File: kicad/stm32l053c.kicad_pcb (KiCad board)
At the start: 2 copper layers, 52 x 35 mm, 42 parts, among them P1 SWD, P2 PWR, Q1 BC807, Q2 BC817, SW1 SW_PUSH, SW2 SW_PUSH, SW3 SW_PUSH, U1 STM32L053C8_LQFP48, U2 TLV61225, U3 um66t, Y1 Crystal

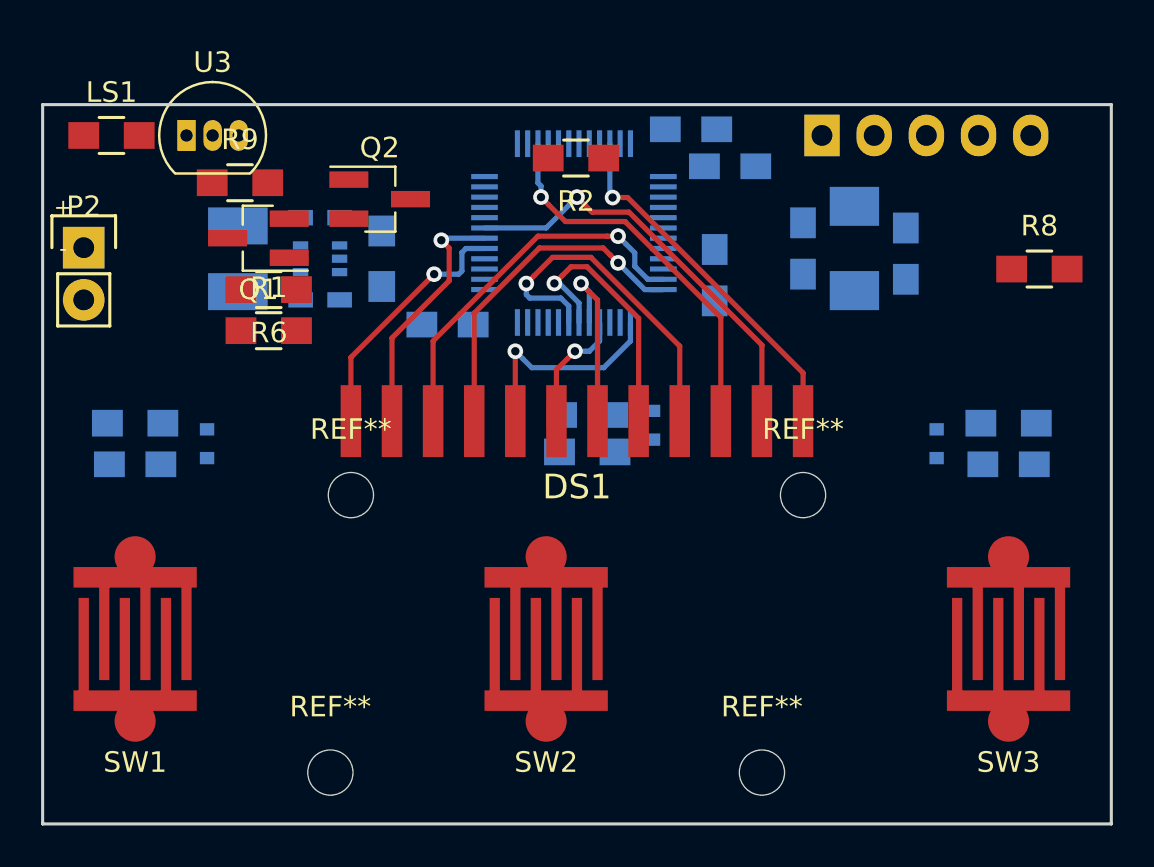
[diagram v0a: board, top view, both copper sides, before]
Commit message: Crystal & melody footprints
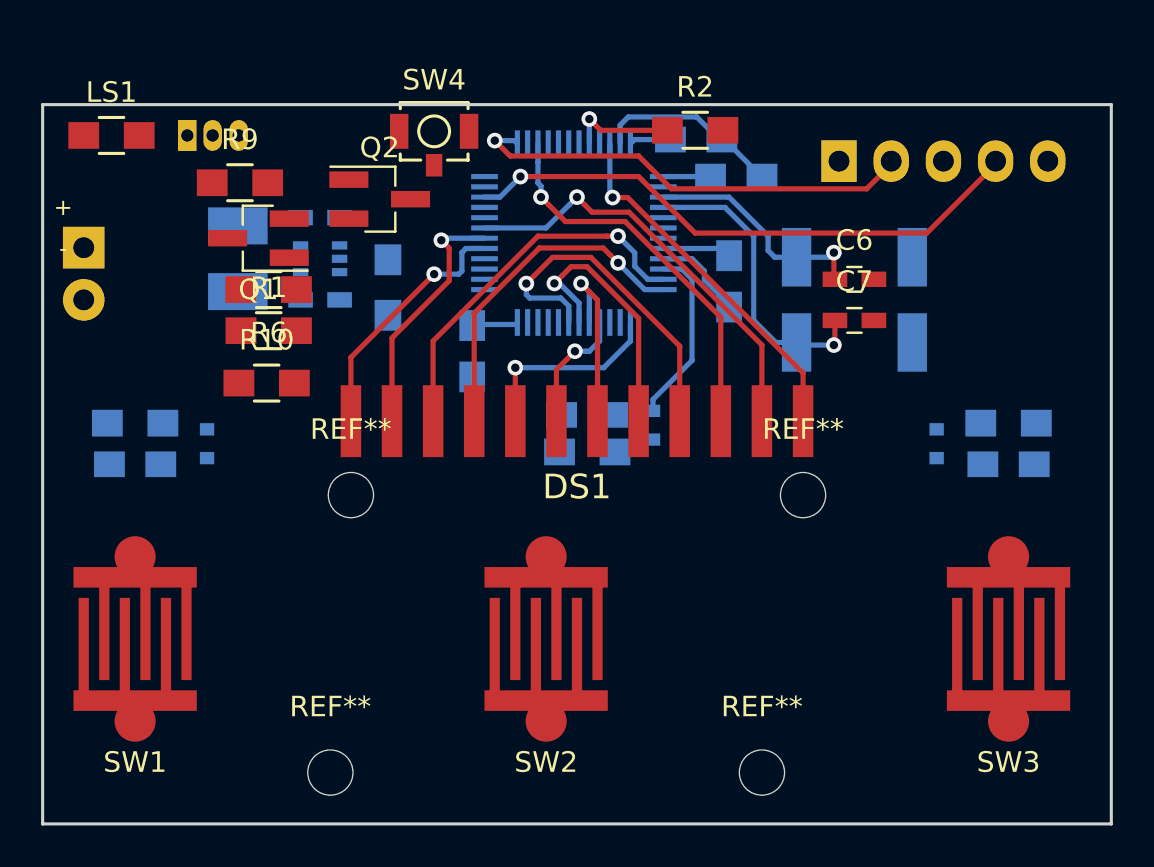
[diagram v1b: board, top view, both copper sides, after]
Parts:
- removed R8: 0, Resistors_SMD:R_0805_HandSoldering
- added R10: 2K2, Resistors_SMD:R_0805_HandSoldering, F.Cu at (127.9, 99.2)
- added SW4: SW_SPDT, Buttons_Switches_SMD:SW_SPST_B3U-1100P, F.Cu at (136.1, 86.9)
- C6, C7: value 20pF -> 4.3pF; footprint Capacitors_SMD:C_0805_HandSoldering -> Capacitors_SMD:C_0603_HandSoldering; moved to F.Cu
- P2: moved to B.Cu
- U3: footprint TO_SOT_Packages_THT:TO-92_Inline_Narrow_Oval -> theapi:UM66T_MELODY; moved to B.Cu
- Y1: value Crystal -> Crystal_GND23; footprint Crystals:ABM3 -> Crystals:Crystal_SMD_SeikoEpson_MC306-4pin_8.0x3.2mm_HandSoldering
- moved R2 5.96 mm to (148.8, 86.8), turned to 0 degrees
- moved C7 4.10 mm to (156.5, 96.1), turned to 0 degrees
- moved C6 2.92 mm to (156.5, 94.1), turned to 0 degrees
- moved U3 2.54 mm to (126.5, 87.1), turned to 180 degrees
- moved Y1 2.50 mm to (156.5, 95.1), turned to 0 degrees
- moved C2 1.77 mm to (137.9, 97.6), turned to 270 degrees
- moved P1 1.50 mm to (155.8, 88.3)
- moved R7 1.43 mm to (133.8, 94.5)
- moved C3 0.76 mm to (150.4, 94.2)
- moved C4 0.58 mm to (150.8, 89.1)
- moved C1 0.56 mm to (148.8, 87.3)
- turned P2 to 180 degrees
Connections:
- C3 pad 1: /VDDA -> VDD
- R9 pad 2: /NPN_BASE -> Net-(R9-Pad2)
- U1 pad 14: Net-(U1-Pad14) -> (no net)
- U1 pad 15: PA5 -> (no net)
- U1 pad 2: Net-(U1-Pad2) -> (no net)
- U1 pad 20: Net-(U1-Pad20) -> (no net)
- U1 pad 21: Net-(U1-Pad21) -> (no net)
- U1 pad 26: Net-(U1-Pad26) -> (no net)
- U1 pad 27: Net-(U1-Pad27) -> (no net)
- U1 pad 28: Net-(U1-Pad28) -> (no net)
- U1 pad 32: Net-(U1-Pad32) -> (no net)
- U1 pad 33: Net-(U1-Pad33) -> (no net)
- U1 pad 38: Net-(U1-Pad38) -> (no net)
- U1 pad 43: Net-(U1-Pad43) -> (no net)
- U1 pad 45: Net-(U1-Pad45) -> (no net)
- U1 pad 5: Net-(U1-Pad5) -> (no net)
- U1 pad 6: Net-(U1-Pad6) -> (no net)
- U1 pad 9: /VDDA -> VDD
- Y1 pad 1: /OSC32_OUT -> /OSC32_IN
- Y1 pad 2: /OSC32_IN -> (no net)
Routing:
- net SWDIO: track 0.00 -> 28.0 mm, vias 0 -> 1
- net SWCLK: track 0.00 -> 22.4 mm, vias 0 -> 1
- net /OSC32_OUT: track 0.00 -> 14.7 mm, vias 0 -> 1
- net Earth: track 0.00 -> 12.5 mm
- net /OSC32_IN: track 0.00 -> 11.3 mm, vias 0 -> 1
- net /WAKEUP_PIN1: track 0.00 -> 8.80 mm
- net VDD: track 0.00 -> 8.72 mm
- net Net-(R2-Pad1): track 0.00 -> 5.23 mm, vias 0 -> 1
- net /VLCD: track 0.00 -> 2.30 mm
- net /LCD_SEG2: track 12.0 -> 10.9 mm
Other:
- board text added: "SWDIO"
- board text removed: "DIO"
